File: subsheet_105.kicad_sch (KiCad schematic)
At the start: 7 parts, among them U10 MC68000_DIP_64_PHY

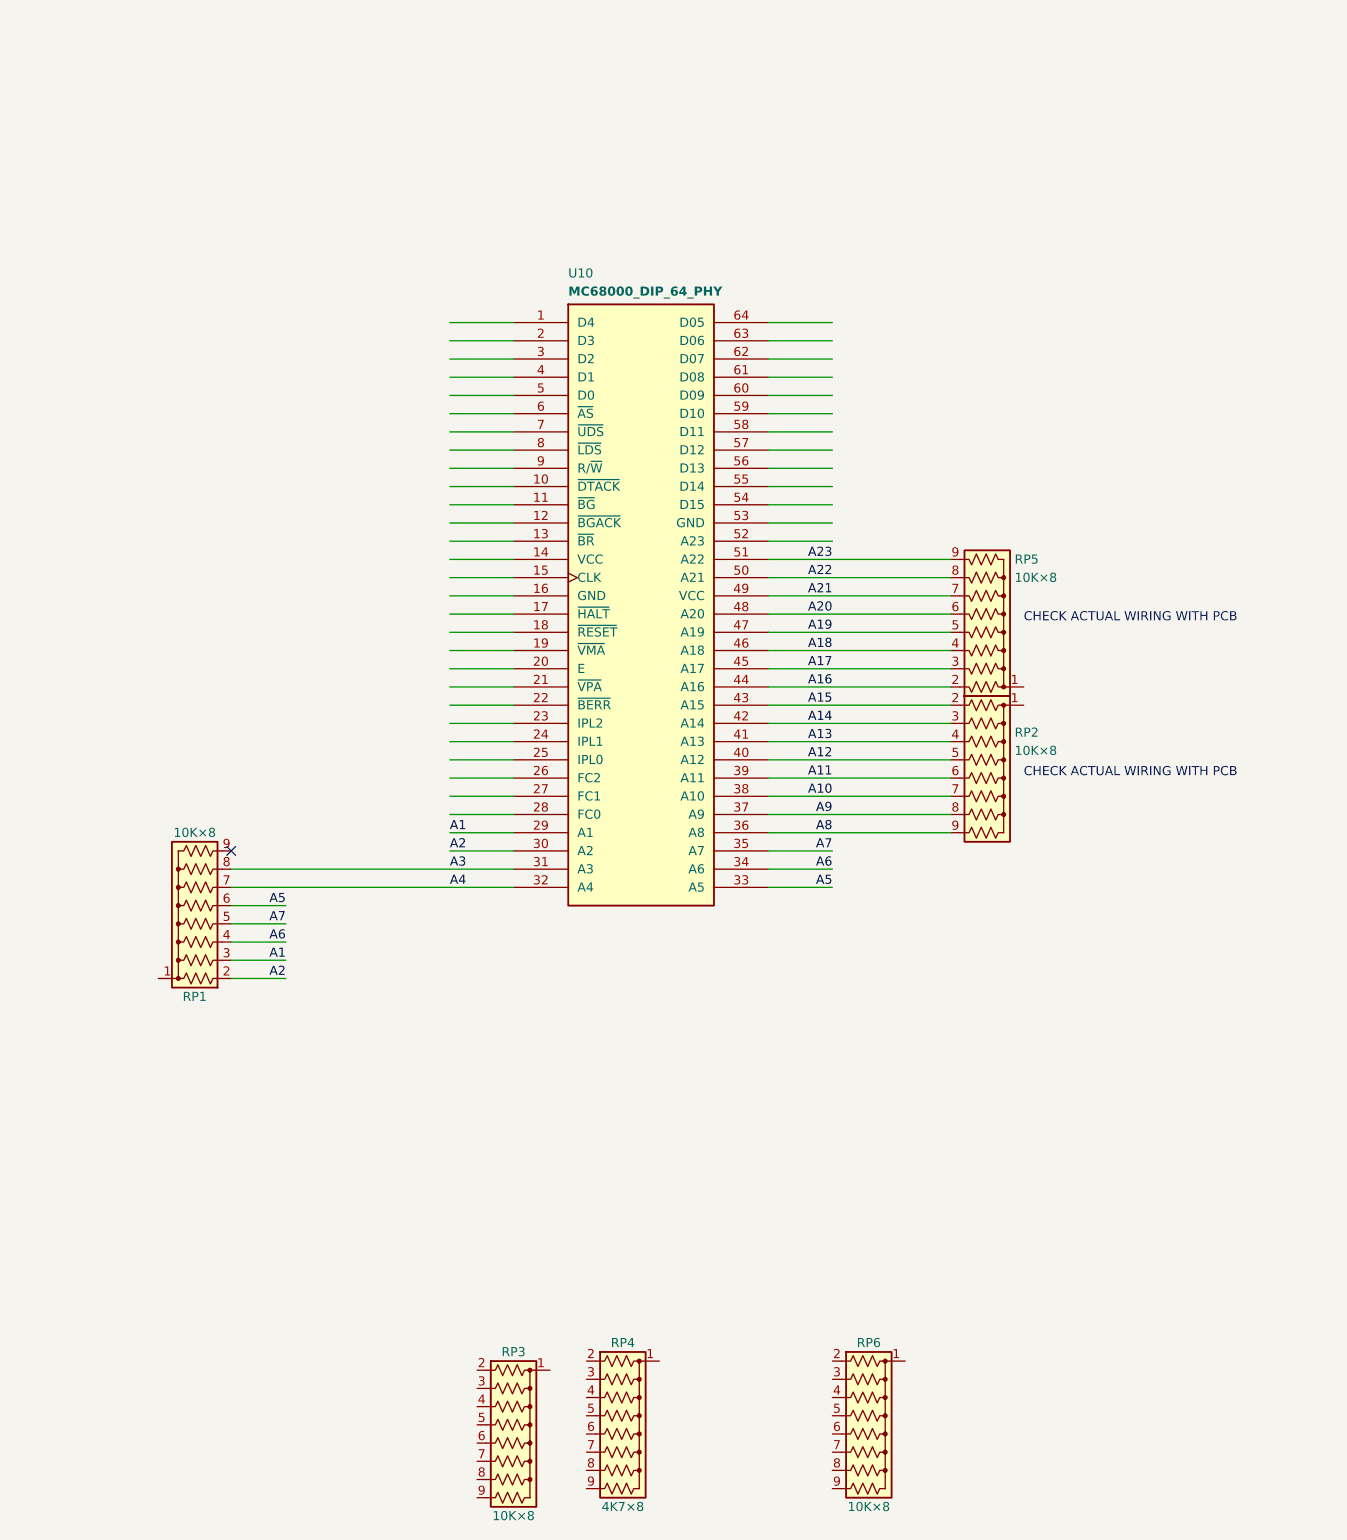
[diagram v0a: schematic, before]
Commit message: continue CPU : some resistor networks, power supply, buses
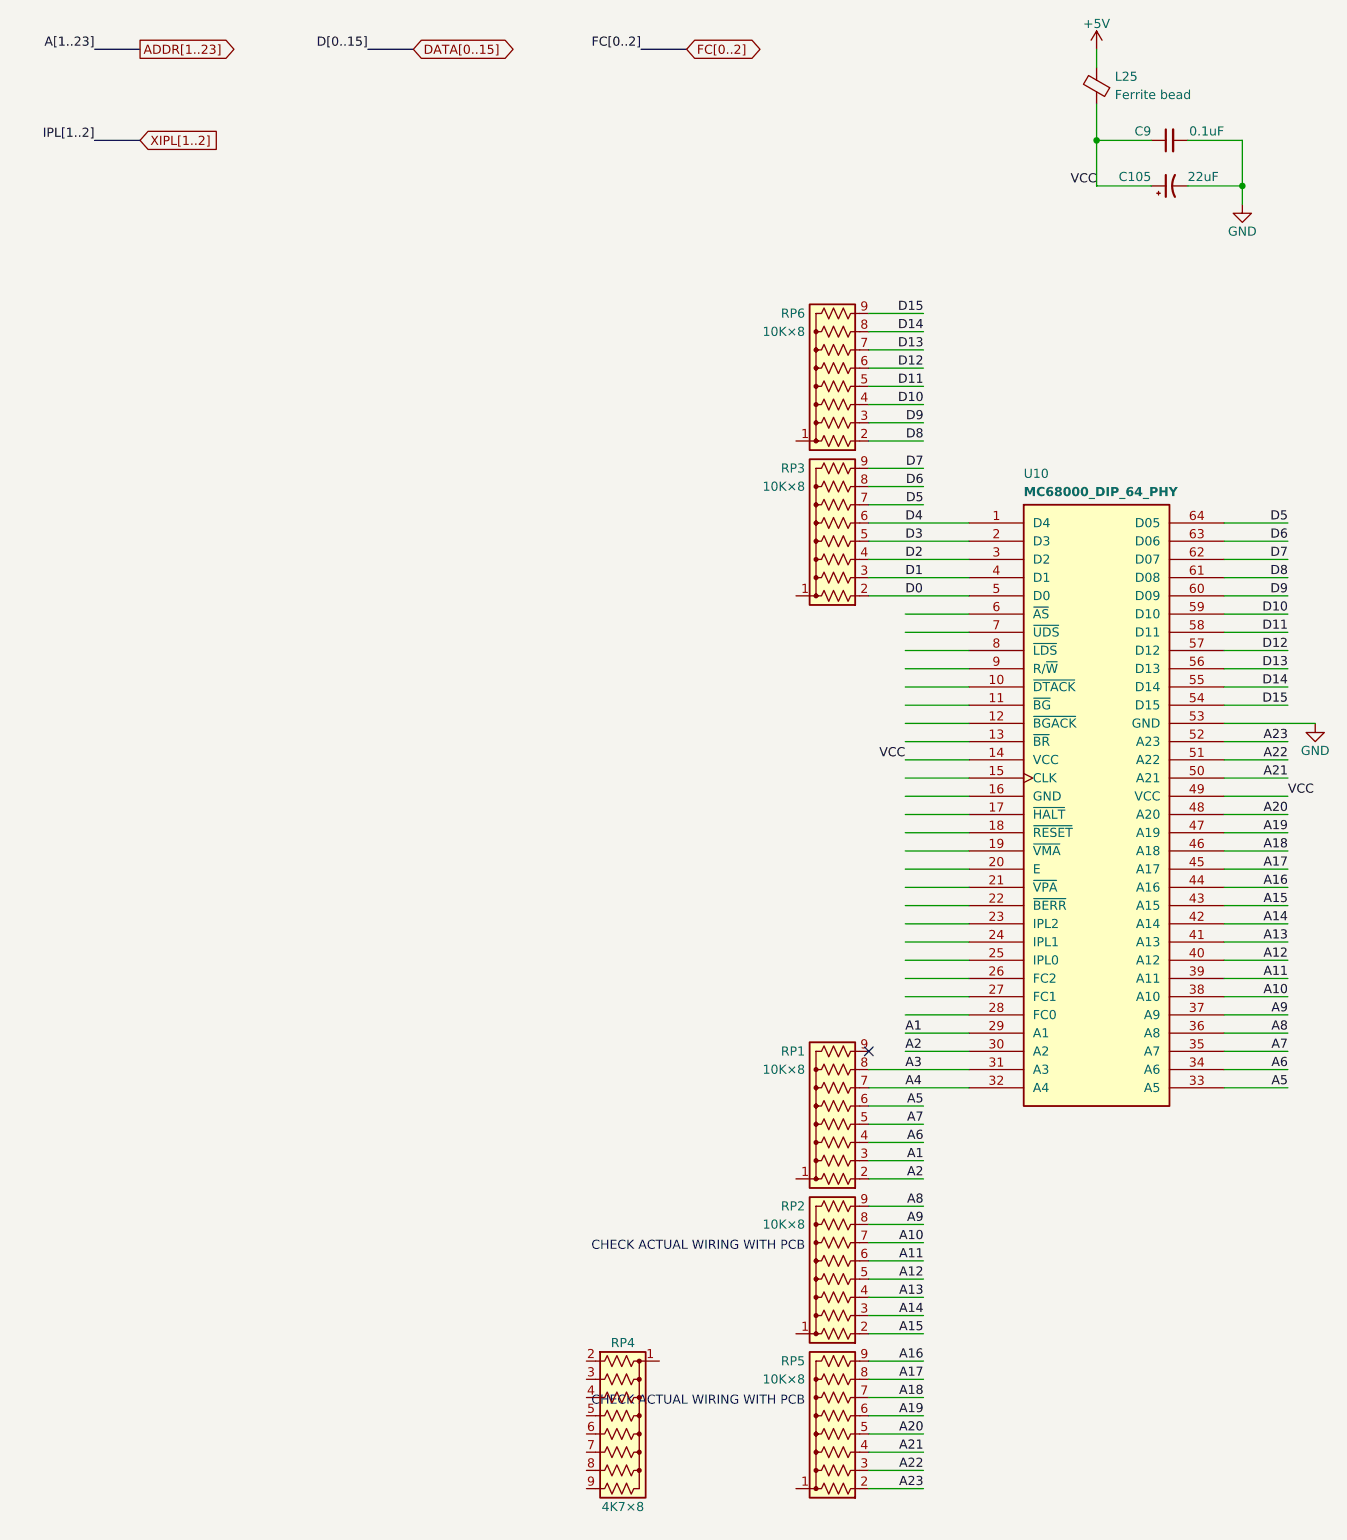
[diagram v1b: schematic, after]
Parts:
- added C105: 22uF, symbol Device:C_Polarized_Small_US
- added C9: 0.1uF, commons-passives_THT:Passive_THT_capacitor_mlcc_W2.54mm_L12.70mm, symbol Device:C_Small
- added L25: Ferrite bead, commons-passives_THT:Passive_THT_ferrite_bead_W3.81mm_L15.24mm, symbol Device:Ferrite_Bead_Small
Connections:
- net A16: now also RP5.9 (R8); no longer RP5.2 (R1)
- net A17: now also RP5.8 (R7); no longer RP5.3 (R2)
- net A18: now also RP5.7 (R6); no longer RP5.4 (R3)
- net A19: now also RP5.6 (R5); no longer RP5.5 (R4)
- net A20: now also RP5.5 (R4); no longer RP5.6 (R5)
- net A21: now also RP5.4 (R3), U10.50 (A21); no longer RP5.7 (R6), U10.49 (VCC)
- net A22: now also RP5.3 (R2), U10.51 (A22); no longer RP5.8 (R7), U10.50 (A21)
- net A23: now also RP5.2 (R1), U10.52 (A23); no longer RP5.9 (R8), U10.51 (A22)
- net D4: now reaches U10.1 (D4)
- net D4: now also RP3.6 (R5)
- net VCC: now reaches U10.14 (VCC)
- net VCC: now also U10.49 (VCC), C105.1, C9.1, L25.1
- net D3: now reaches U10.2 (D3)
- net D3: now also RP3.5 (R4)
- net D2: now reaches U10.3 (D2)
- net D2: now also RP3.4 (R3)
- net D1: now reaches U10.4 (D1)
- net D1: now also RP3.3 (R2)
- net D0: now reaches U10.5 (D0)
- net D0: now also RP3.2 (R1)
- net GND: now reaches U10.53 (GND)
- net GND: now also C105.2, C9.2
- net D15: now reaches U10.54 (D15)
- net D15: now also RP6.9 (R8)
- net D14: now reaches U10.55 (D14)
- net D14: now also RP6.8 (R7)
- net D13: now reaches U10.56 (D13)
- net D13: now also RP6.7 (R6)
- net D12: now reaches U10.57 (D12)
- net D12: now also RP6.6 (R5)
- net D11: now reaches U10.58 (D11)
- net D11: now also RP6.5 (R4)
- net D10: now reaches U10.59 (D10)
- net D10: now also RP6.4 (R3)
- net D9: now reaches U10.60 (D09)
- net D9: now also RP6.3 (R2)
- net D8: now reaches U10.61 (D08)
- net D8: now also RP6.2 (R1)
- net D7: now reaches U10.62 (D07)
- net D7: now also RP3.9 (R8)
- net D6: now reaches U10.63 (D06)
- net D6: now also RP3.8 (R7)
- net D5: now reaches U10.64 (D05)
- net D5: now also RP3.7 (R6)
- new net +5V: L25.2
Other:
- moved on the sheet: RP1, RP2, RP3, RP5, RP6, U10
